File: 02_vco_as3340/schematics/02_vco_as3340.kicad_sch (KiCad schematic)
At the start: 89 parts, among them J1 Header 1, J10 SINE OUT, J2 Header 2, J3 SYNC IN, J4 FM IN, J5 PWM CV IN, J6 1V per O IN, J7 SQUARE OUT, J8 SAW OUT, J9 TRI OUT, Q1 BC547C, Q2 BC547C, U1 TL072, U2 AS3340, U3 TL074

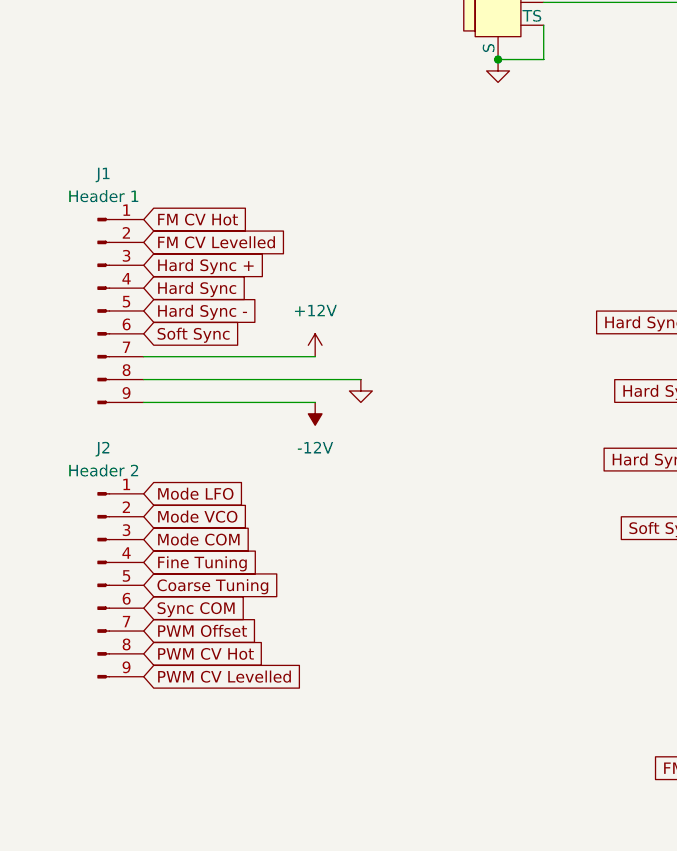
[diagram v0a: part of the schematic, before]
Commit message: routed everyting
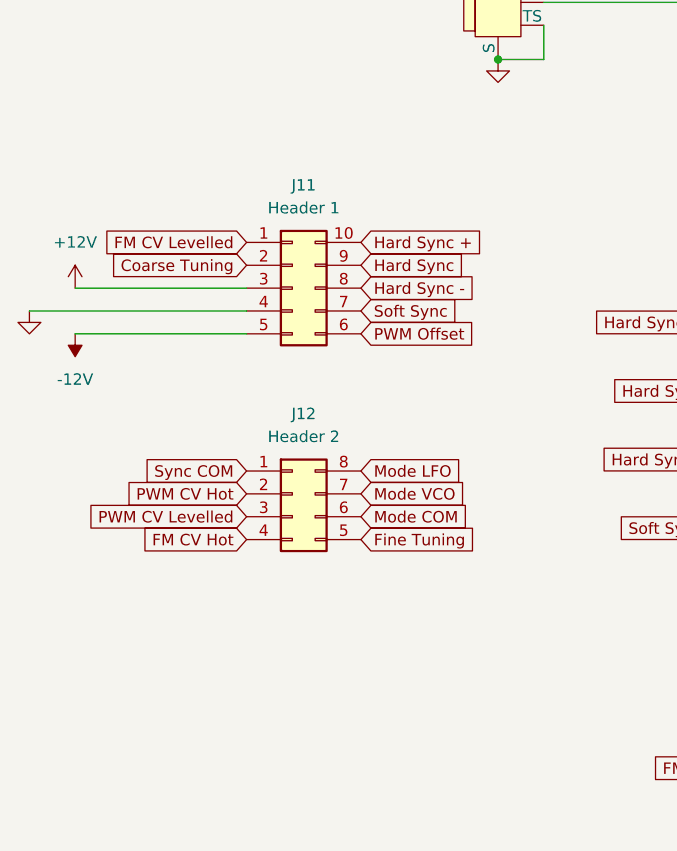
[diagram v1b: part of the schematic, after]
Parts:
- removed J1: Header 1, Connector_PinHeader_2.54mm:PinHeader_1x09_P2.54mm_Vertical, symbol Connector:Conn_01x09_Pin
- removed J2: Header 2, Connector_PinHeader_2.54mm:PinHeader_1x09_P2.54mm_Vertical, symbol Connector:Conn_01x09_Pin
- added J11: Header 1, Connector_PinSocket_2.54mm:PinSocket_2x05_P2.54mm_Vertical, symbol Connector_Generic:Conn_02x05_Counter_Clockwise
- added J12: Header 2, Connector_PinSocket_2.54mm:PinSocket_2x04_P2.54mm_Vertical, symbol Connector_Generic:Conn_02x04_Counter_Clockwise
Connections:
- net +12V: now also J11.3 (Pin_3)
- net -12V: now also J11.5 (Pin_5)
- net Coarse Tuning: now also J11.2 (Pin_2)
- net FM CV Hot: now also J12.4 (Pin_4)
- net FM CV Levelled: now also J11.1 (Pin_1)
- net Fine Tuning: now also J12.5 (Pin_5)
- net GND: now also J11.4 (Pin_4)
- net Hard Sync: now also J11.9 (Pin_9)
- net Hard Sync +: now also J11.10 (Pin_10)
- net Hard Sync -: now also J11.8 (Pin_8)
- net Mode COM: now also J12.6 (Pin_6)
- net Mode LFO: now also J12.8 (Pin_8)
- net Mode VCO: now also J12.7 (Pin_7)
- net PWM CV Hot: now also J12.2 (Pin_2)
- net PWM CV Levelled: now also J12.3 (Pin_3)
- net PWM Offset: now also J11.6 (Pin_6)
- net Soft Sync: now also J11.7 (Pin_7)
- net Sync COM: now also J12.1 (Pin_1)
